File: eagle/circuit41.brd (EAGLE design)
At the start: 47 x 71.2 mm, 18 parts

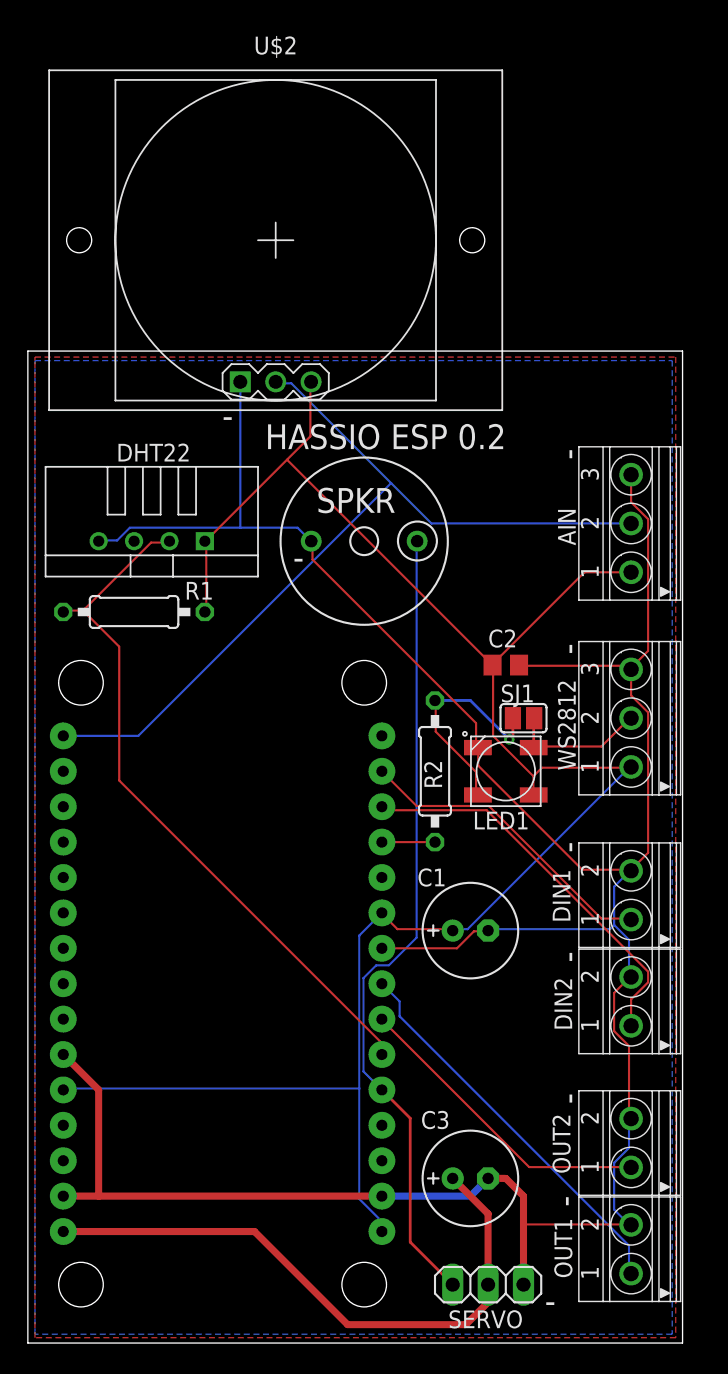
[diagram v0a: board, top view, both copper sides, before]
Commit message: main update to version 0.41
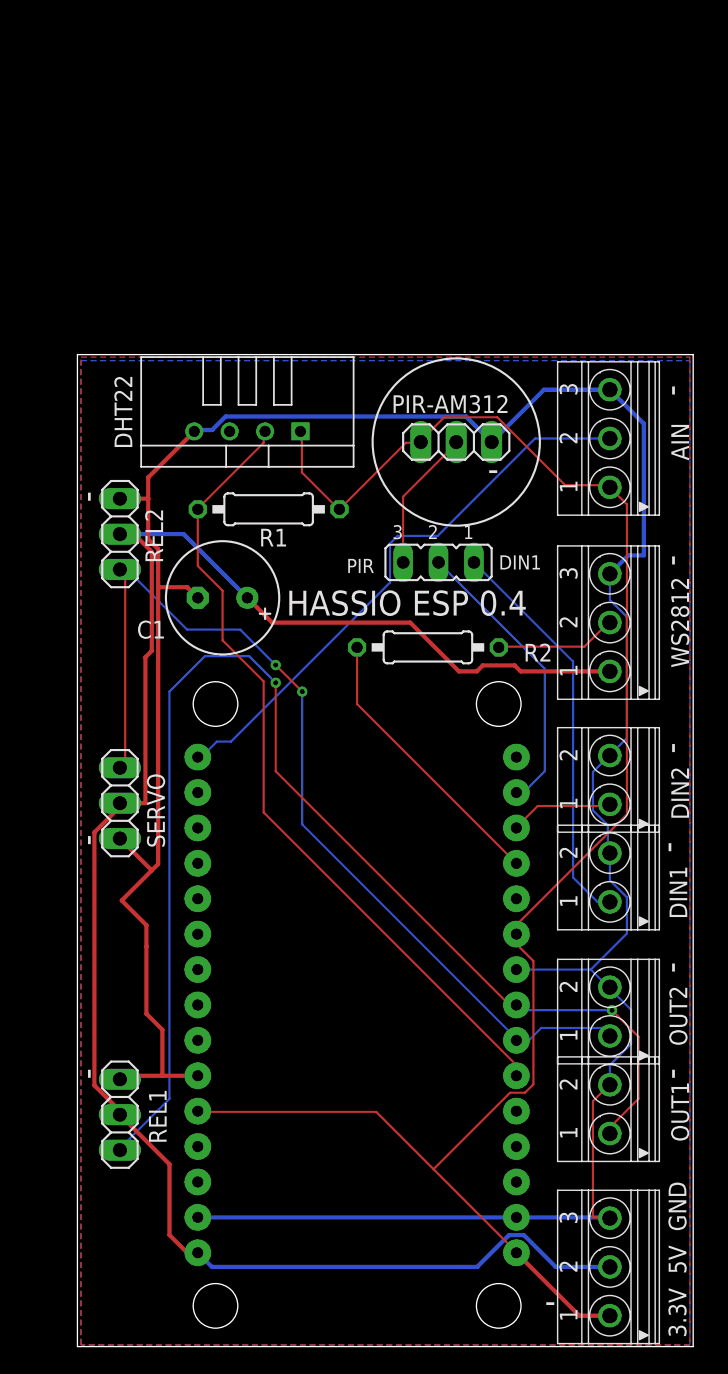
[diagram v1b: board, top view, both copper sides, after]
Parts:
- removed C2: 100n, rcl:C0805
- removed C3: (no value), rcl:E2,5-7
- removed LED1: WS2812B, WS2812B:WS2812B
- removed SJ1: (no value), jumper:SJ
- removed SPKR: BMT1205XH7.5, buzzer:BMT1205XH7.5
- removed U$2: MOTION-PIR-DYP-ME003, diy-modules:MOTION-PIR-DYP-ME003
- added JP3: (no value), jumper:JP2
- added PIR-AM312, REL1, REL2: (no value), pinhead:1X03
- added PWR: 1751251, con-phoenix-350:1751251
- C1: value (none) -> 1000uF; device rcl:E2,5-7 -> rcl:E3,5-8
- R2: value (none) -> 470
- moved SERVO 43.5 mm to (6.60, 37.1), turned to 270 degrees
- moved C1 29.8 mm to (14.0, 51.8), turned to 180 degrees
- moved DIN2 16.0 mm to (41.7, 38.8)
- moved R1 12.1 mm to (17.3, 58.2)
- moved DHT22 10.4 mm to (15.7, 63.8)
- moved OUT1 10.2 mm to (41.7, 15.1)
- moved U$1 9.77 mm to (23.6, 22.6)
- moved OUT2 9.55 mm to (41.7, 22.1)
- moved R2 8.90 mm to (28.7, 48.3), turned to 0 degrees
- moved WS2812 7.03 mm to (41.7, 50.0)
- moved AIN 6.28 mm to (41.7, 63.2)
- moved DIN1 1.98 mm to (41.7, 31.8)
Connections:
- removed net N$5: OUT1.1, U$1.D5
- removed net N$7: OUT2.1, U$1.D6
- removed net N$9: DIN1.1, U$1.D1
- removed net WS: LED1.DIN, R2.2, SJ1.1
- new net N$2: DIN1.1, JP3.1
- new net PIR-DATA: JP3.3, PIR-AM312.2
- new net RELOUT1: OUT1.1, REL1.3, U$1.D5
- new net RELOUT2: OUT2.1, REL2.3, SERVO.1, U$1.D6
- net ANALOGIN: no longer U$2.2
- net DOUT: now also R2.2; no longer LED1.DOUT, SJ1.2
- net GND: now also PIR-AM312.3, PWR.3, REL1.1, REL2.1; no longer C2.2, C3.-, LED1.VSS, SPKR.-, U$2.1
- net N$1: now also JP3.2, U$1.D1; no longer SERVO.1, SPKR.+, U$1.D8
- net VCC: now also PIR-AM312.1, PWR.1; no longer C1.+, C2.1, LED1.VDD, U$2.3, WS2812.1
- net VIN: now also C1.+, PWR.2, REL1.2, REL2.2, WS2812.1; no longer C3.+
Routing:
- net RELOUT1: track 0.00 -> 92.4 mm, vias 0 -> 2
- net VIN: track 43.9 -> 131.0 mm
- net RELOUT2: track 0.00 -> 70.3 mm, vias 0 -> 2
- net N$1: track 58.1 -> 20.8 mm
- net N$2: track 0.00 -> 28.9 mm
- net N$5: track 28.3 -> 0.00 mm
- net N$7: track 22.3 -> 0.00 mm
- net N$9: track 22.3 -> 0.00 mm
- net N$11: track 28.4 -> 7.43 mm
- net ANALOGIN: track 60.8 -> 40.7 mm
- net WS-DATA: track 3.81 -> 20.2 mm
- net WS: track 16.2 -> 0.00 mm, vias 1 -> 0
- net VCC: track 140.1 -> 124.2 mm
- net PIR-DATA: track 0.00 -> 10.6 mm
- net DHT-DATA: track 50.5 -> 57.9 mm
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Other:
- board size 47 x 71.2 mm -> 44.2 x 71.2 mm
- board text added: "3.3V 5V GND"
- board text added: "DIN1"
- board text added: "HASSIO ESP 0.4"
- board text added: "PIR"
- board text removed: "HASSIO ESP 0.2"
